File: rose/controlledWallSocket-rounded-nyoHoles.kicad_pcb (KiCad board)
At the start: 2 copper layers, 85.6 x 85.6 mm, 93 parts, among them J1 screw term. 2x1 5mm, J10 IDC 6x2, J11 IDC 2x2, J12 IDC 2x2, J13 pinHeader 7x1 2.54mm, J14 pinHeader 4x1 2.54mm, J15 Conn_01x08_Pin, J2 screw term. 2x1 5mm, J3 USB_TypeC, J4 sdCard_DM3AT-SF-PEJM5, J5 IDC 2x2, J6 IDC 2x2, J7 IDC 2x2, J8 IDC 6x2, J9 IDC 2x2, M1 RTC and EEPROM, Q1 bc337, Q2 BSS138, Q3 BSS138, Q4 bc337, SW1 SW_Push, SW2 SW_Push, SW3 SW_Push, SW4 SW_Push, U1 LM66100Q, U2 LM66100Q, U3 LM66100Q, U4 LM66100Q, U5 USBLC6-2SC6, U6 LM66100Q, U7 TPS565242DRLR, U8 ESP32-S3-WROOM-1

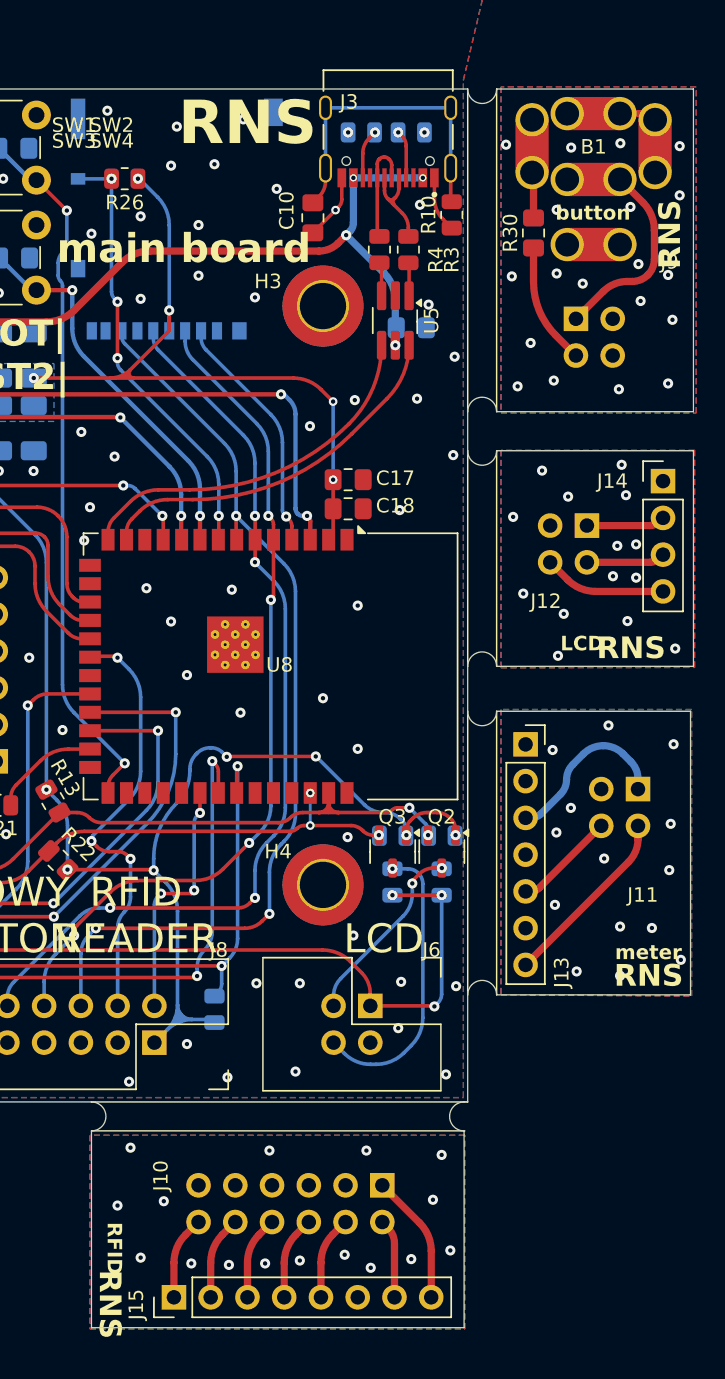
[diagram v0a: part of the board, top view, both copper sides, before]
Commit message: knop guiater update
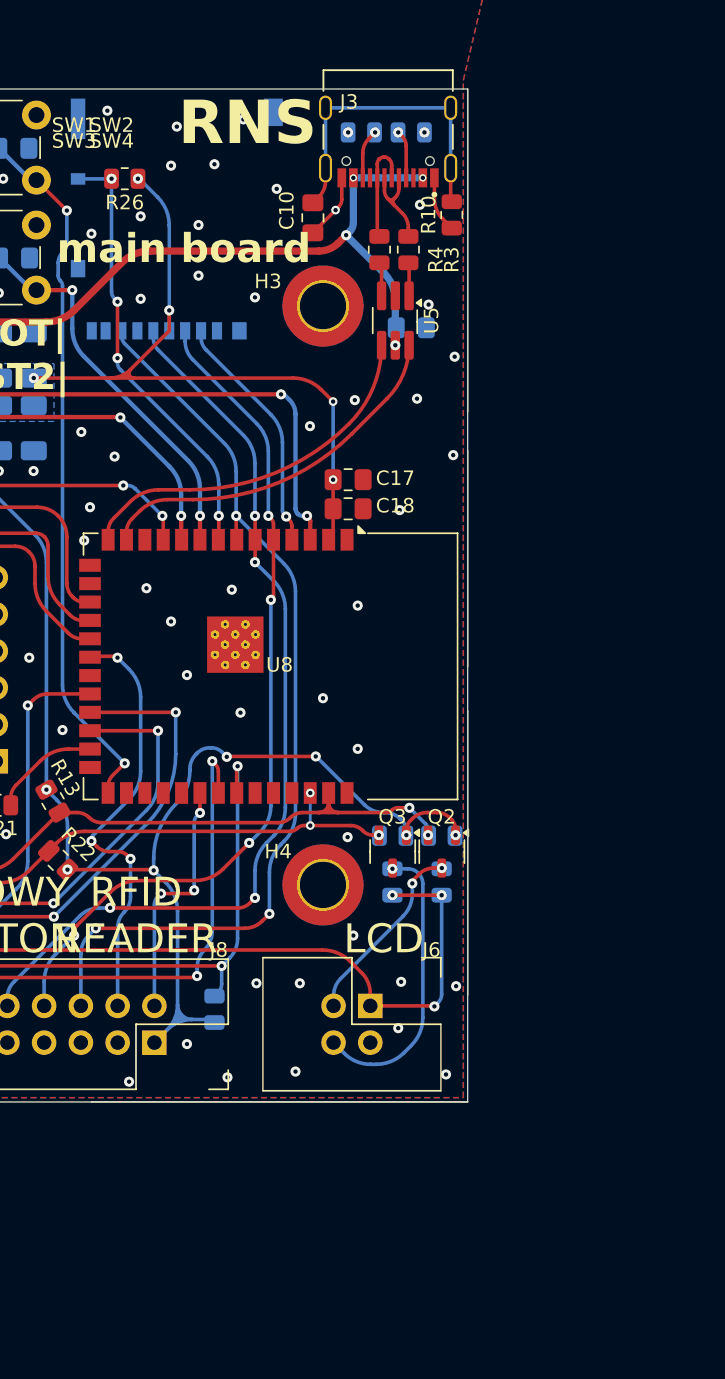
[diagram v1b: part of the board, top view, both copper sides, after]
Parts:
- removed B1: Button, customStuff:button
- removed J10: IDC 6x2, customStuff:IDC 6x2 2.54
- removed J11, J12, J9: IDC 2x2, customStuff:IDC 2x2 2.54
- removed J13: pinHeader 7x1 2.54mm, Connector_PinSocket_2.54mm:PinSocket_1x07_P2.54mm_Vertical
- removed J14: pinHeader 4x1 2.54mm, Connector_PinHeader_2.54mm:PinHeader_1x04_P2.54mm_Vertical
- removed J15: Conn_01x08_Pin, Connector_PinHeader_2.54mm:PinHeader_1x08_P2.54mm_Vertical
- removed R30: 100R, Capacitor_SMD:C_0805_2012Metric_Pad1.18x1.45mm_HandSolder
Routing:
- net bG_button: track 13.8 -> 0.00 mm
- net Net-(J11-Pin_2): track 12.7 -> 0.00 mm
- net Net-(J11-Pin_1): track 12.2 -> 0.00 mm
- net Net-(J10-Pin_1): track 9.02 -> 0.00 mm
- net Net-(J12-Pin_4): track 8.50 -> 0.00 mm
- net bG_LED: track 8.40 -> 0.00 mm
- net Net-(J11-Pin_4): track 7.07 -> 0.00 mm
- net Net-(J10-Pin_4): track 5.77 -> 0.00 mm
- net Net-(J10-Pin_8): track 5.77 -> 0.00 mm
- net Net-(J10-Pin_6): track 5.77 -> 0.00 mm
- net Net-(J10-Pin_10): track 5.77 -> 0.00 mm
- net Net-(J10-Pin_12): track 5.77 -> 0.00 mm
- net Net-(J10-Pin_2): track 5.49 -> 0.00 mm
- net Net-(J12-Pin_2): track 5.44 -> 0.00 mm
- net Net-(J12-Pin_1): track 5.44 -> 0.00 mm
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- removed copper zone on B.Cu, net Net-(J10-Pin_11)
- removed copper zone on F.Cu, net Net-(J10-Pin_11)
- removed copper zone on B.Cu, net Net-(J11-Pin_3)
- removed copper zone on F.Cu, net Net-(J11-Pin_3)
- removed copper zone on B.Cu, net Net-(J12-Pin_3)
- removed copper zone on F.Cu, net Net-(J12-Pin_3)
- removed copper zone on B.Cu, net bG_GND
- removed copper zone on F.Cu, net bG_GND
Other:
- board size 85.6 x 85.6 mm -> 70 x 70 mm
- board text removed: "RFID"
- board text removed: "button"
- board text removed: "meter"
